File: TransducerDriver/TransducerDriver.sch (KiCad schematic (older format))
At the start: 53 parts, among them J1 ModSigJack, J2 BattJack+, J3 BattJack-, Q3 IRF540N, Q4 IRF540N, T1 Transformer_SP_1S 1:10, T2 Transformer_SP_1S 1:10, T3 Transformer_SP_1S 1:10, U1 TL082, U2 INA217-Amplifier_Instrumentat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, U3 TC427, U4 LM4562, Y1 Crystal, Y2 Fish Finder, Y3 FishFinder, Y4 FishFinder

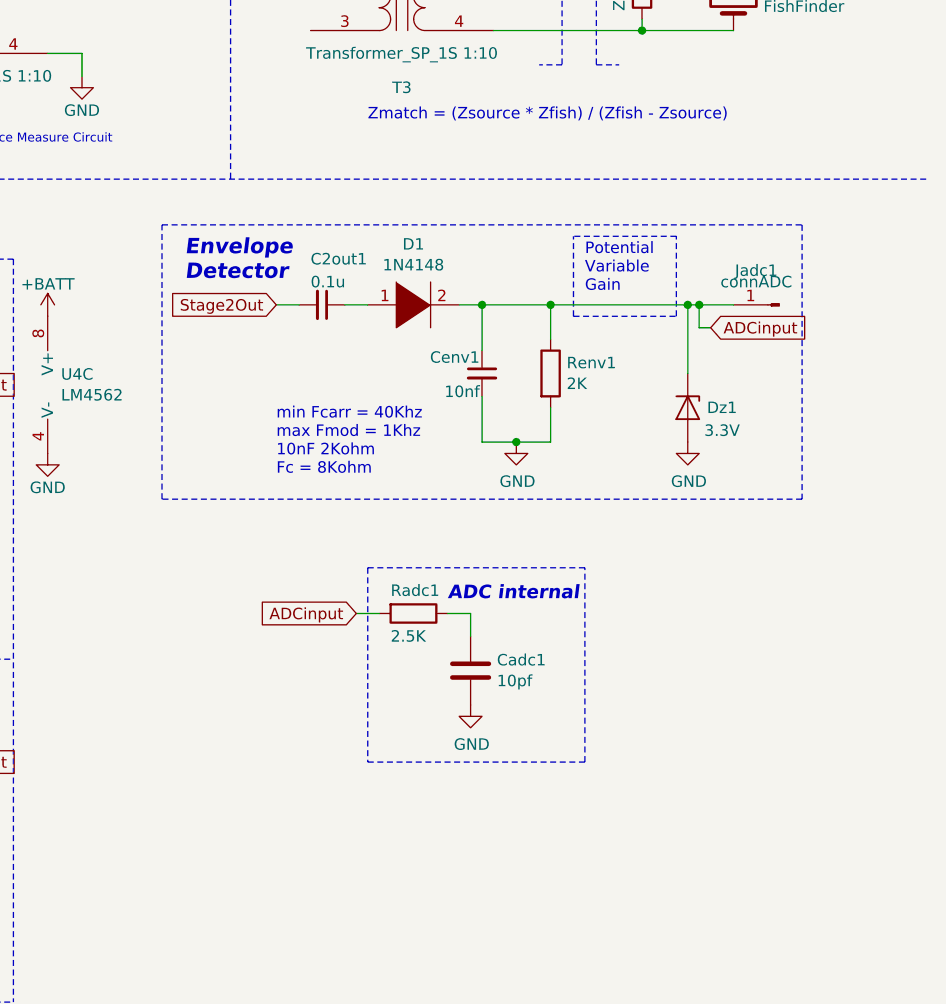
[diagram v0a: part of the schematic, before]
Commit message: more mod on circuits
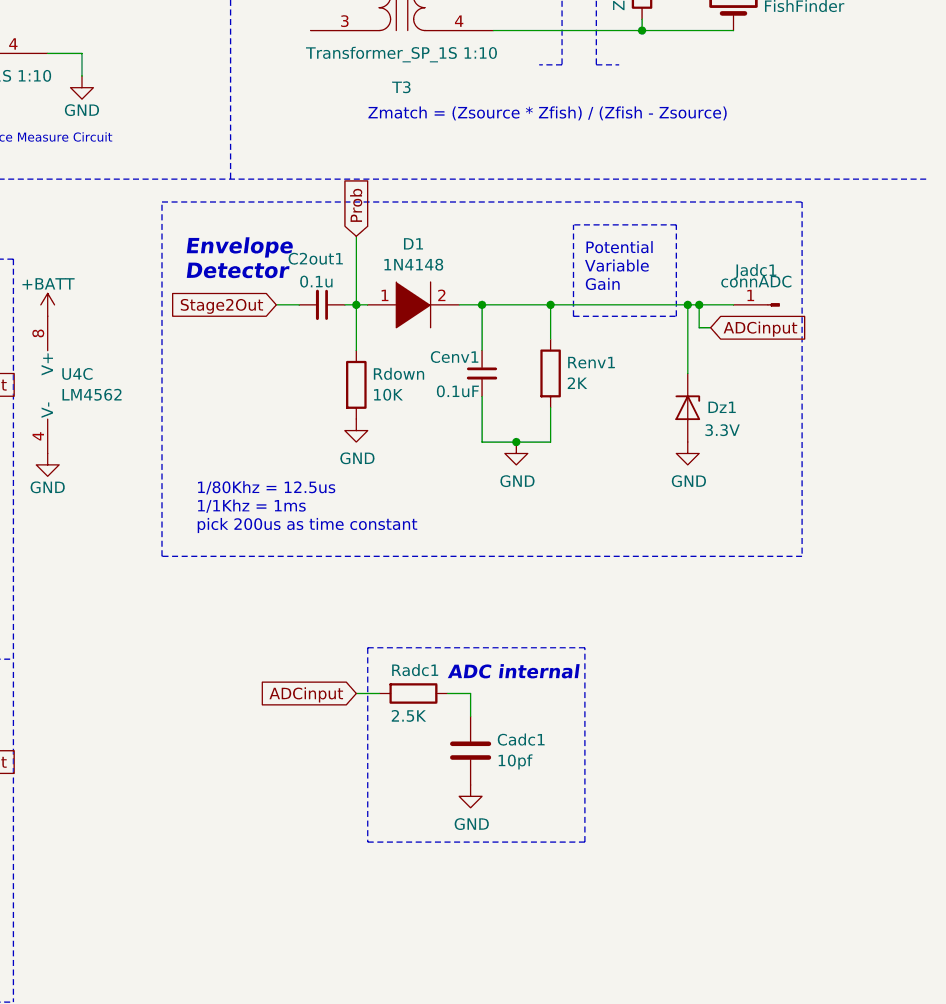
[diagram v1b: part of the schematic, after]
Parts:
- added Rdown: 10K, Resistors_THT:R_Axial_DIN0309_L9.0mm_D3.2mm_P12.70mm_Horizontal, symbol Device:R
- Cenv1: value 10nf -> 0.1uF
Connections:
- net GND: now also Rdown.2
- net Prob: now reaches C2out1.1, D1.1 (K)
- net Prob: now also Rdown.1
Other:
- note added: "1/80Khz = 12.5us\n1/1Khz = 1ms\npick 200us as time constant"
- note removed: "min Fcarr = 40Khz \nmax Fmod = 1Khz \n10nF 2Kohm\nFc = 8Kohm"
- moved on the sheet: Cadc1, Radc1
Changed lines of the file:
@@
 	2200 2200 1900 2200
-Wire Wire Line
-	3500 2000 3600 2000
 Wire Wire Line
 	3600 2000 3600 1800
@@
 Wire Wire Line
 	10150 4100 10150 3800
-Text GLabel 8700 5150 0    50   Input ~ 0
+Text GLabel 8700 5500 0    50   Input ~ 0
 ADCinput
 $Comp
 L Device:R Radc1
 U 1 1 5E653FDE
-P 8950 5150
-F 0 "Radc1" V 8850 5050 50  0000 L CNN
-F 1 "2.5K" V 9050 5050 50  0000 L CNN
-F 2 "Resistors_THT:R_Axial_DIN0309_L9.0mm_D3.2mm_P12.70mm_Horizontal" V 8880 5150 50  0001 C CNN
-F 3 "~" H 8950 5150 50  0001 C CNN
-	1    8950 5150
+P 8950 5500
+F 0 "Radc1" V 8850 5400 50  0000 L CNN
+F 1 "2.5K" V 9050 5400 50  0000 L CNN
+F 2 "Resistors_THT:R_Axial_DIN0309_L9.0mm_D3.2mm_P12.70mm_Horizontal" V 8880 5500 50  0001 C CNN
+F 3 "~" H 8950 5500 50  0001 C CNN
+	1    8950 5500
 	0    1    1    0
 $EndComp
@@
 L Device:C Cadc1
 U 1 1 5E654634
-P 9200 5400
-F 0 "Cadc1" H 9085 5354 50  0000 R CNN
-F 1 "10pf" H 9085 5445 50  0000 R CNN
-F 2 "Capacitors_THT:C_Disc_D8.0mm_W5.0mm_P7.50mm" H 9238 5250 50  0001 C CNN
-F 3 "~" H 9200 5400 50  0001 C CNN
-	1    9200 5400
+P 9200 5750
+F 0 "Cadc1" H 9085 5704 50  0000 R CNN
+F 1 "10pf" H 9085 5795 50  0000 R CNN
+F 2 "Capacitors_THT:C_Disc_D8.0mm_W5.0mm_P7.50mm" H 9238 5600 50  0001 C CNN
+F 3 "~" H 9200 5750 50  0001 C CNN
+	1    9200 5750
 	-1   0    0    1
 $EndComp
 Wire Wire Line
-	9100 5150 9200 5150
-Wire Wire Line
-	9200 5150 9200 5250
-Wire Wire Line
-	8800 5150 8700 5150
+	9100 5500 9200 5500
+Wire Wire Line
+	9200 5500 9200 5600
+Wire Wire Line
+	8800 5500 8700 5500
 $Comp
 L power:GND #PWR012
 U 1 1 5E65CE66
-P 9200 5550
-F 0 "#PWR012" H 9200 5300 50  0001 C CNN
-F 1 "GND" H 9205 5377 50  0000 C CNN
-F 2 "" H 9200 5550 50  0001 C CNN
-F 3 "" H 9200 5550 50  0001 C CNN
-	1    9200 5550
-	1    0    0    -1
-$EndComp
-Wire Notes Line
-	8750 4950 8750 5800
-Wire Notes Line
-	8750 5800 9700 5800
-Wire Notes Line
-	9700 5800 9700 4950
-Wire Notes Line
-	9700 4950 8750 4950
-Text Notes 9100 5100 0    59   Italic 12
+P 9200 5900
+F 0 "#PWR012" H 9200 5650 50  0001 C CNN
+F 1 "GND" H 9205 5727 50  0000 C CNN
+F 2 "" H 9200 5900 50  0001 C CNN
+F 3 "" H 9200 5900 50  0001 C CNN
+	1    9200 5900
+	1    0    0    -1
+$EndComp
+Wire Notes Line
+	8750 5300 8750 6150
+Wire Notes Line
+	8750 6150 9700 6150
+Wire Notes Line
+	9700 6150 9700 5300
+Wire Notes Line
+	9700 5300 8750 5300
+Text Notes 9100 5450 0    59   Italic 12
 ADC internal
-$Comp
-L Device:C_Small Cenv1
-U 1 1 5E672EB5
-P 9250 4100
-F 0 "Cenv1" H 9260 4170 50  0000 L CNN
-F 1 "10nf" H 9260 4020 50  0000 L CNN
-F 2 "Capacitors_THT:C_Disc_D5.0mm_W2.5mm_P5.00mm" H 9250 4100 50  0001 C CNN
-F 3 "~" H 9250 4100 50  0001 C CNN
-	1    9250 4100
-	-1   0    0    -1
-$EndComp
 Wire Wire Line
 	9250 3800 9250 4000
@@
 U 1 1 5E67C655
 P 8550 3800
-F 0 "C2out1" V 8750 3750 50  0000 L CNN
-F 1 "0.1u" V 8650 3750 50  0000 L CNN
+F 0 "C2out1" V 8750 3650 50  0000 L CNN
+F 1 "0.1u" V 8650 3700 50  0000 L CNN
 F 2 "Capacitors_THT:C_Disc_D5.0mm_W2.5mm_P5.00mm" H 8550 3800 50  0001 C CNN
 F 3 "~" H 8550 3800 50  0001 C CNN
@@
 	0    1    -1   0
 $EndComp
-Text Notes 8350 4550 0    50   ~ 0
-min Fcarr = 40Khz \nmax Fmod = 1Khz \n10nF 2Kohm\nFc = 8Kohm
 Wire Wire Line
 	8350 3800 8450 3800
 Wire Wire Line
-	8650 3800 8750 3800
+	8650 3800 8700 3800
 Wire Notes Line
 	9650 3850 10100 3850
 Wire Notes Line
-	10100 3850 10100 3500
-Wire Notes Line
-	10100 3500 9650 3500
-Wire Notes Line
-	9650 3850 9650 3500
+	10100 3850 10100 3450
+Wire Notes Line
+	10100 3450 9650 3450
+Wire Notes Line
+	9650 3850 9650 3450
 Text Notes 9700 3750 0    50   ~ 0
 Potential\nVariable \nGain
-Wire Wire Line
-	9250 3800 9550 3800
 Wire Wire Line
 	9550 3800 10150 3800
@@
 Envelope\nDetector
 Wire Notes Line
-	7850 3450 10650 3450
-Wire Notes Line
-	10650 3450 10650 4650
-Wire Notes Line
-	10650 4650 7850 4650
-Wire Notes Line
-	7850 4650 7850 3450
+	7850 3350 10650 3350
+Wire Notes Line
+	10650 3350 10650 4900
+Wire Notes Line
+	10650 4900 7850 4900
+Wire Notes Line
+	7850 4900 7850 3350
 $Comp
 L Connector:Conn_01x01_Male Jadc1
@@
 	3200 3700 3550 3700
 Wire Wire Line
-	5300 1850 5600 1850
-Wire Wire Line
 	5300 2250 5600 2250
 Text GLabel 2000 4400 0    50   Input ~ 0
@@
 Text Notes 8200 700  0    157  ~ 31
 Impedance Match
+Wire Wire Line
+	3500 2000 3600 2000
+Wire Wire Line
+	5300 1850 5600 1850
+$Comp
+L Device:C_Small Cenv1
+U 1 1 5E672EB5
+P 9250 4100
+F 0 "Cenv1" H 9260 4170 50  0000 L CNN
+F 1 "0.1uF" H 9260 4020 50  0000 L CNN
+F 2 "Capacitors_THT:C_Disc_D5.0mm_W2.5mm_P5.00mm" H 9250 4100 50  0001 C CNN
+F 3 "~" H 9250 4100 50  0001 C CNN
+	1    9250 4100
+	-1   0    0    -1
+$EndComp
+Text Notes 8000 4800 0    50   ~ 0
+1/80Khz = 12.5us\n1/1Khz = 1ms\npick 200us as time constant
+$Comp
+L Device:R Rdown
+U 1 1 5E5726AC
+P 8700 4150
+F 0 "Rdown" H 8770 4196 50  0000 L CNN
+F 1 "10K" H 8770 4105 50  0000 L CNN
+F 2 "Resistors_THT:R_Axial_DIN0309_L9.0mm_D3.2mm_P12.70mm_Horizontal" V 8630 4150 50  0001 C CNN
+F 3 "~" H 8700 4150 50  0001 C CNN
+	1    8700 4150
+	1    0    0    -1
+$EndComp
+$Comp
+L power:GND #PWR?
+U 1 1 5E57295E
+P 8700 4300
+F 0 "#PWR?" H 8700 4050 50  0001 C CNN
+F 1 "GND" H 8705 4127 50  0000 C CNN
+F 2 "" H 8700 4300 50  0001 C CNN
+F 3 "" H 8700 4300 50  0001 C CNN
+	1    8700 4300
+	1    0    0    -1
+$EndComp
+Wire Wire Line
+	8700 3800 8700 4000
+Connection ~ 8700 3800
+Wire Wire Line
+	8700 3800 8750 3800
+Text GLabel 8700 3500 1    50   Input ~ 0
+Prob
+Wire Wire Line
+	9250 3800 9550 3800
+Wire Wire Line
+	8700 3500 8700 3800
 $EndSCHEMATC
